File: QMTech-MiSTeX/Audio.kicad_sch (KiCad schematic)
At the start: 16 parts, among them CN1 PJ-327A 5JJ, J9 Conn_01x06_Male, U5 ZGY133/T10(PLT)

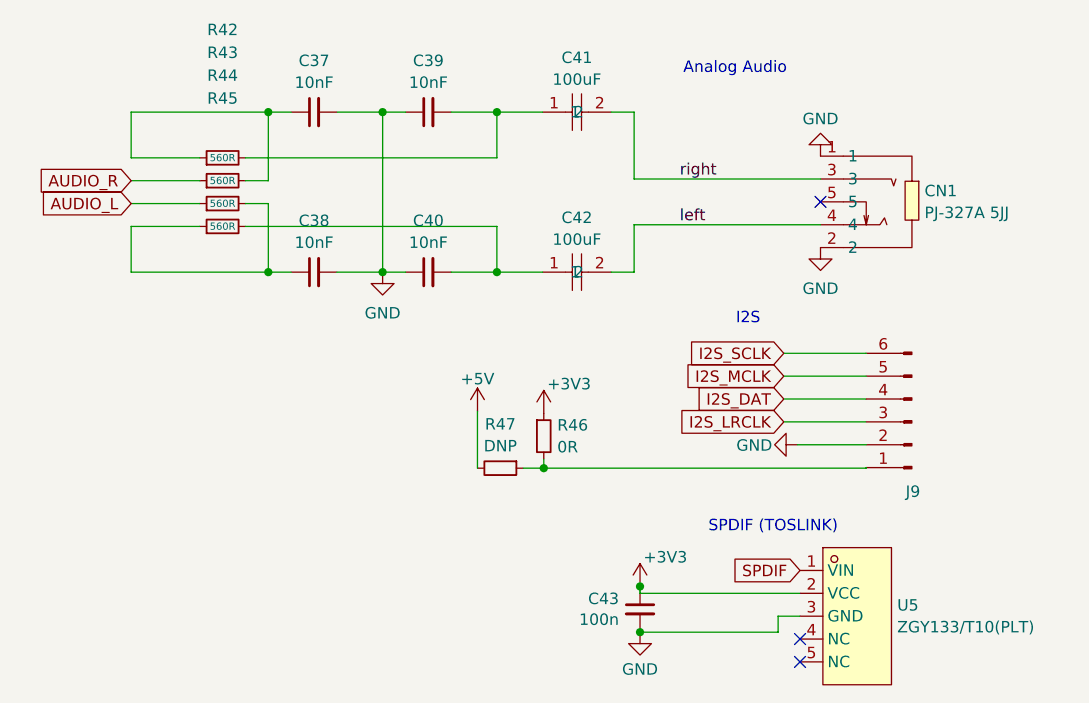
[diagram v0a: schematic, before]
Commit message: QMTech-MiSTeX WIP
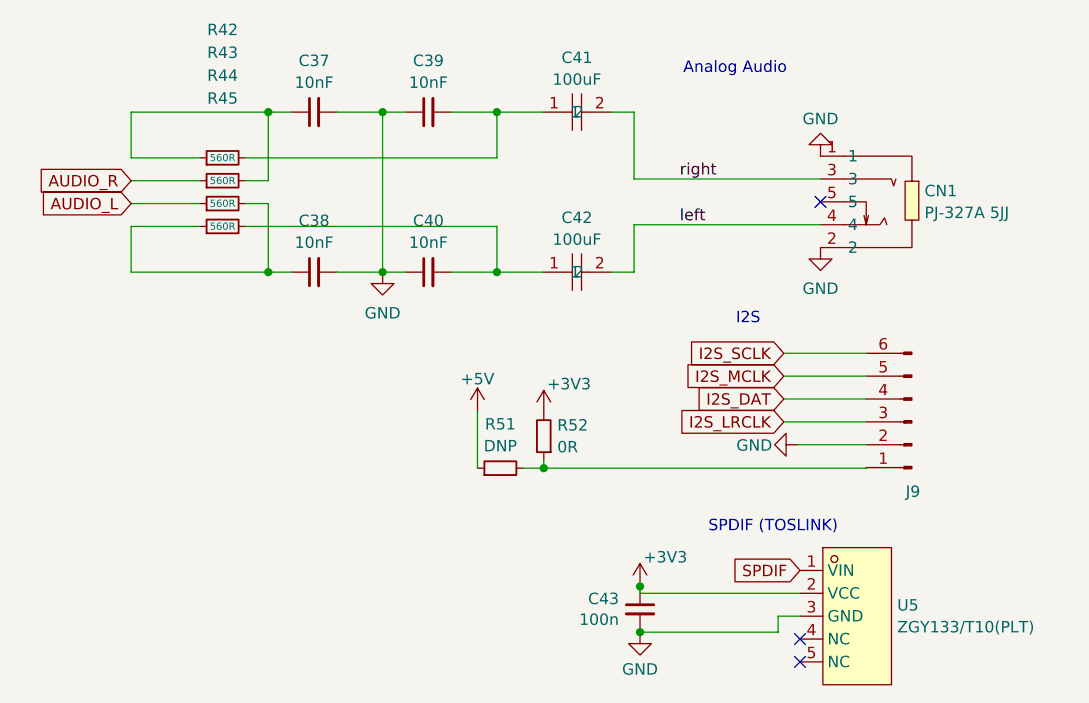
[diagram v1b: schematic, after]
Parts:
- removed R46: 0R, R_0402_1005Metric, symbol jlcpcb-basic-resistor-0402:0R
- removed R47: DNP, R_0402_1005Metric, symbol jlcpcb-basic-resistor-0402:0R
- added R51: DNP, R_0603_1608Metric, symbol jlcpcb-basic-resistor-0603:0R
- added R52: 0R, R_0603_1608Metric, symbol jlcpcb-basic-resistor-0603:0R
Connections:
- net +3V3: now also R52.2
- net +5V: now also R51.1
- net at J9.1 (Pin_1): now also R51.2, R52.1
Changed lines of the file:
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@@
-    )
-  )
-  (symbol (lib_id "jlcpcb-basic-resistor-0402:0R") (at 151.384 119.6987 270) (unit 1)
-    (in_bom yes) (on_board yes) (dnp no) (fields_autoplaced)
-    (property "Reference" "R47" (at 151.384 114.8178 90)
-      (effects (font (size 1.27 1.27)))
-    )
-    (property "Value" "DNP" (at 151.384 117.242 90)
-      (effects (font (size 1.27 1.27)))
-    )
-    (property "Footprint" "R_0402_1005Metric" (at 151.384 117.9207 90)
-      (effects (font (size 1.27 1.27)) hide)
-    )
-    (property "Datasheet" "" (at 151.384 119.6987 90)
-      (effects (font (size 1.27 1.27)) hide)
-    )
-    (pin "1")
-    (pin "2")
-    (instances
-      (project "Audio"
-        (path "/40894532-c7c4-4c7b-a6a8-096cd4259f73"
-          (reference "R47") (unit 1)
-        )
-      )
-      (project "QMTech-MiSTeX"
-        (path "/bf95850e-2fcb-4784-a603-f17fc357556b/1e65a514-c552-4463-908f-afe88949be5c"
-          (reference "R51") (unit 1)
-        )
-      )
     )
   )
@@
     )
   )
-  (symbol (lib_id "jlcpcb-basic-resistor-0402:0R") (at 156.21 116.1427 0) (unit 1)
-    (in_bom yes) (on_board yes) (dnp no) (fields_autoplaced)
-    (property "Reference" "R46" (at 157.7086 114.9306 0)
-      (effects (font (size 1.27 1.27)) (justify left))
-    )
-    (property "Value" "0R" (at 157.7086 117.3548 0)
-      (effects (font (size 1.27 1.27)) (justify left))
-    )
-    (property "Footprint" "R_0402_1005Metric" (at 154.432 116.1427 90)
-      (effects (font (size 1.27 1.27)) hide)
-    )
-    (property "Datasheet" "https://datasheet.lcsc.com/szlcsc/Uniroyal-Elec-0402WGF0000TCE_C17168.pdf" (at 156.21 116.1427 90)
-      (effects (font (size 1.27 1.27)) hide)
-    )
-    (property "LCSC" "C17168" (at 156.21 116.1427 90)
-      (effects (font (size 1.27 1.27)) hide)
-    )
-    (pin "1")
-    (pin "2")
-    (instances
-      (project "Audio"
-        (path "/40894532-c7c4-4c7b-a6a8-096cd4259f73"
-          (reference "R46") (unit 1)
-        )
-      )
-      (project "QMTech-MiSTeX"
-        (path "/bf95850e-2fcb-4784-a603-f17fc357556b/1e65a514-c552-4463-908f-afe88949be5c"
-          (reference "R52") (unit 1)
-        )
-      )
-    )
-  )
   (symbol (lib_id "jlcpcb-basic-resistor-0603:560R") (at 120.523 87.757 90) (unit 1)
     (in_bom yes) (on_board yes) (dnp no)
@@
     )
   )
+  (symbol (lib_id "jlcpcb-basic-resistor-0603:0R") (at 156.21 116.1427 180) (unit 1)
+    (in_bom yes) (on_board yes) (dnp no) (fields_autoplaced)
+    (property "Reference" "R52" (at 157.7086 114.9306 0)
+      (effects (font (size 1.27 1.27)) (justify right))
+    )
+    (property "Value" "0R" (at 157.7086 117.3548 0)
+      (effects (font (size 1.27 1.27)) (justify right))
+    )
+    (property "Footprint" "R_0603_1608Metric" (at 157.988 116.1427 90)
+      (effects (font (size 1.27 1.27)) hide)
+    )
+    (property "Datasheet" "https://datasheet.lcsc.com/szlcsc/Uniroyal-Elec-0603WAF0000T5E_C21189.pdf" (at 156.21 116.1427 90)
+      (effects (font (size 1.27 1.27)) hide)
+    )
+    (property "LCSC" "C21189" (at 156.21 116.1427 90)
+      (effects (font (size 1.27 1.27)) hide)
+    )
+    (pin "2")
+    (pin "1")
+    (instances
+      (project "QMTech-MiSTeX"
+        (path "/bf95850e-2fcb-4784-a603-f17fc357556b/1e65a514-c552-4463-908f-afe88949be5c"
+          (reference "R52") (unit 1)
+        )
+      )
+    )
+  )
   (symbol (lib_id "power:GND") (at 184.404 117.094 270) (mirror x) (unit 1)
     (in_bom yes) (on_board yes) (dnp no)
@@
         )
       )
+    )
+  )
+  (symbol (lib_id "jlcpcb-basic-resistor-0603:0R") (at 151.384 119.6987 90) (unit 1)
+    (in_bom yes) (on_board yes) (dnp no) (fields_autoplaced)
+    (property "Reference" "R51" (at 151.384 114.8178 90)
+      (effects (font (size 1.27 1.27)))
+    )
+    (property "Value" "DNP" (at 151.384 117.242 90)
+      (effects (font (size 1.27 1.27)))
+    )
+    (property "Footprint" "R_0603_1608Metric" (at 151.384 121.4767 90)
+      (effects (font (size 1.27 1.27)) hide)
+    )
+    (property "Datasheet" "https://datasheet.lcsc.com/szlcsc/Uniroyal-Elec-0603WAF0000T5E_C21189.pdf" (at 151.384 119.6987 90)
+      (effects (font (size 1.27 1.27)) hide)
+    )
+    (property "LCSC" "C21189" (at 151.384 119.6987 90)
+      (effects (font (size 1.27 1.27)) hide)
+    )
+    (pin "2")
+    (pin "1")
+    (instances
+      (project "QMTech-MiSTeX"
+        (path "/bf95850e-2fcb-4784-a603-f17fc357556b/1e65a514-c552-4463-908f-afe88949be5c"
+          (reference "R51") (unit 1)
+        )
+      )
